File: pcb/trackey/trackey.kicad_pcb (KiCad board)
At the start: 2 copper layers, 55.9 x 77.5 mm, 31 parts, among them J1 trackball_port, J2 Audio-Jack-4, J3 COL_port, J4 ROW_port, J6 has_trackball, J7 is_left, U1 Arduino_Pro_Micro, U2 Arduino_Pro_Micro, U3 MCP23S17

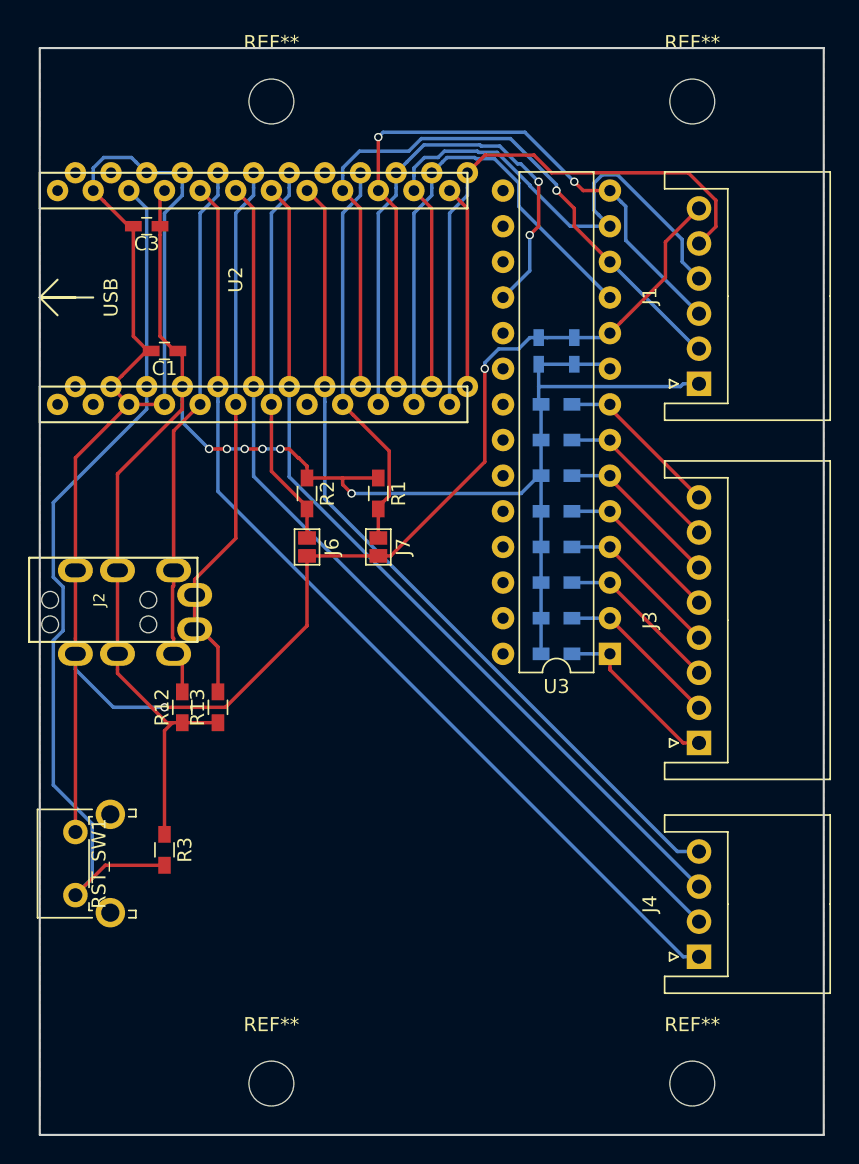
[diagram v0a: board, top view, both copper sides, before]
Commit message: improve pcb size
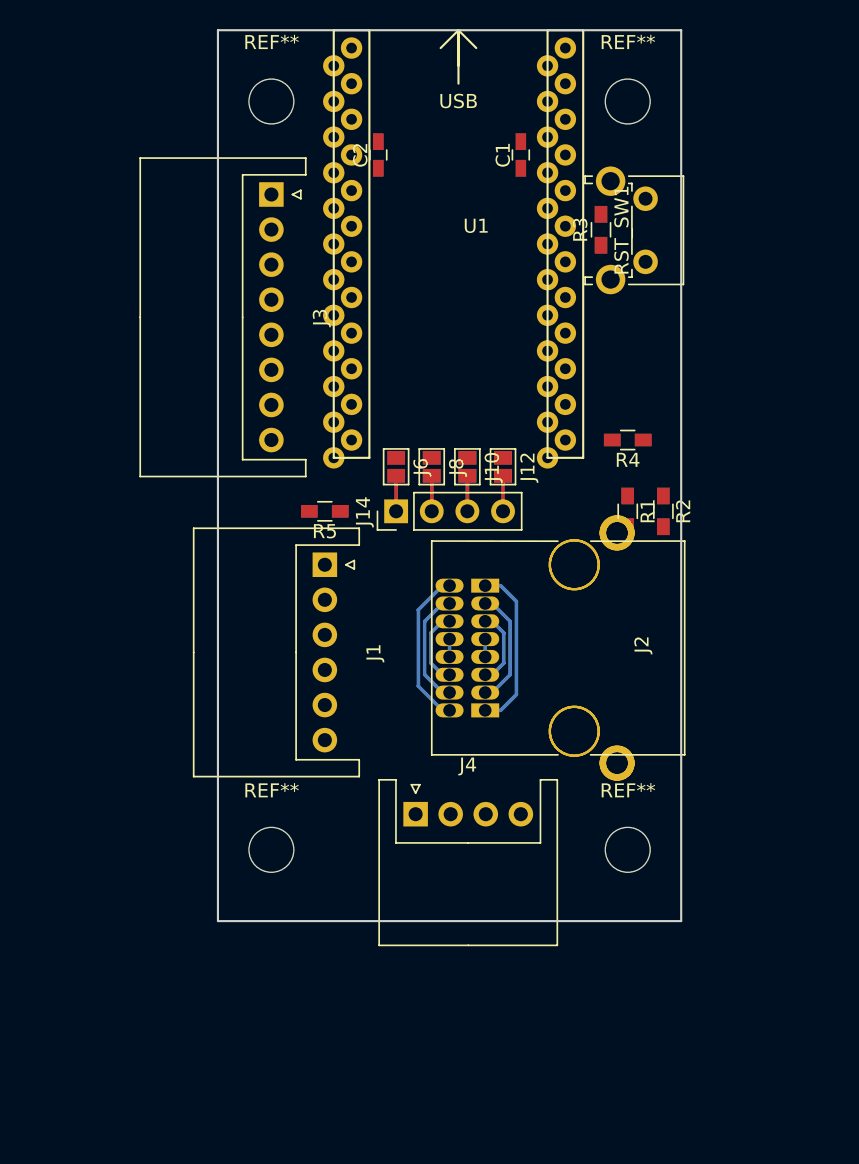
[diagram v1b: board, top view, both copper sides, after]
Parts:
- removed C3: 1uF, Capacitors_SMD:C_0603_HandSoldering
- removed C4: 0.1uF, Capacitors_SMD:C_0603_HandSoldering
- removed R10, R11, R6, R7, R8, R9: 10kΩ, Resistors_SMD:R_0603_HandSoldering
- removed R12, R13: 2.2kΩ, Resistors_SMD:R_0603_HandSoldering
- removed the REF** at (30.0, 0.00)
- removed the REF** at (0.00, 70.0)
- removed the REF** at (30.0, 70.0)
- removed U3: MCP23S17, Housings_DIP:DIP-28_W7.62mm
- added J10: is_left, Connectors:GS2, F.Cu at (14.0, 26.0)
- added J11: is_right, Connectors:GS2, B.Cu at (14.0, 26.0)
- added J12: is_left, Connectors:GS2, F.Cu at (16.5, 26.0)
- added J13: is_right, Connectors:GS2, B.Cu at (16.5, 26.0)
- added J14: OLED_conn, Socket_Strips:Socket_Strip_Straight_1x04_Pitch2.54mm, F.Cu at (8.89, 29.2)
- added J5: RJ45, trackey:RJ45_8, B.Cu at (15.2, 34.5)
- added J8: is_left, Connectors:GS2, F.Cu at (11.4, 26.0)
- added J9: is_right, Connectors:GS2, B.Cu at (11.4, 26.0)
- added REF**: MountingHole_3.2mm_M3, Mounting_Holes:MountingHole_3.2mm_M3, F.Cu at (25.4, 0.00)
- added REF**: MountingHole_3.2mm_M3, Mounting_Holes:MountingHole_3.2mm_M3, F.Cu at (0.00, 53.3)
- added REF**: MountingHole_3.2mm_M3, Mounting_Holes:MountingHole_3.2mm_M3, F.Cu at (25.4, 53.3)
- C2, U1: moved to F.Cu
- J2: value Audio-Jack-4 -> RJ45; footprint trackey:MJ-4PP-9_rev2 -> trackey:RJ45_8
- J6: value has_trackball -> is_left
- J7: value is_left -> is_right; moved to B.Cu
- R1, R2: value 2.2kΩ -> 2.2k
- R4, R5: value 10kΩ -> 2.2k; moved to F.Cu
- U2: moved to B.Cu
- moved RST_SW1 64.2 mm to (26.7, 6.93), turned to 270 degrees
- moved R3 54.1 mm to (23.5, 9.14), turned to 90 degrees
- moved J3 49.6 mm to (0.00, 6.63), turned to 270 degrees
- moved J2 33.5 mm to (15.2, 43.4)
- moved J1 29.6 mm to (3.81, 33.0), turned to 270 degrees
- moved C1 29.0 mm to (17.8, 3.81), turned to 90 degrees
- moved R2 25.4 mm to (27.9, 29.2)
- moved J4 22.6 mm to (10.3, 50.8), turned to 0 degrees
- moved R5 18.2 mm to (3.81, 29.2), turned to 180 degrees
- moved C2 18.1 mm to (7.62, 3.81)
- moved R1 17.8 mm to (25.4, 29.2)
- moved R4 16.1 mm to (25.4, 24.1), turned to 180 degrees
- moved U1 15.1 mm to (14.6, 10.2), turned to 0 degrees
- moved U2 12.1 mm to (10.8, 11.4), turned to 180 degrees
- moved J6 8.54 mm to (8.89, 26.0)
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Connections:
- J2 pad 1: /SCL -> +5V
- J2 pad 3: +5V -> /SCL
- J2 pad 4: GND -> /SCLK
- J3 pad 8: /COL7 -> Net-(J3-Pad8)
- J6 pad 1: /has_trackball -> /SDA
- J6 pad 2: GND -> /OLED_1
- J7 pad 1: /is_left -> GND
- J7 pad 2: GND -> /OLED_1
- R1 pad 2: /is_left -> /SCL
- R2 pad 2: /has_trackball -> /SDA
- R4 pad 2: /COL0 -> Net-(R4-Pad2)
- R5 pad 1: +5V -> GND
- R5 pad 2: /COL1 -> Net-(R5-Pad2)
- U1 pad 1: Net-(U1-Pad1) -> /COL0
- U1 pad 10: /Key_IO_RST -> /COL5
- U1 pad 11: /Key_SS -> /COL6
- U1 pad 13: /Arduino_SS -> Net-(R4-Pad2)
- U1 pad 2: Net-(U1-Pad2) -> /COL1
- U1 pad 7: /has_trackball -> /COL2
- U1 pad 8: Net-(U1-Pad8) -> /COL3
- U1 pad 9: /is_left -> /COL4
- U2 pad 1: Net-(U2-Pad1) -> /COL0
- U2 pad 10: /Key_IO_RST -> /COL5
- U2 pad 11: /Key_SS -> /COL6
- U2 pad 13: /Arduino_SS -> Net-(R5-Pad2)
- U2 pad 2: Net-(U2-Pad2) -> /COL1
- U2 pad 7: /has_trackball -> /COL2
- U2 pad 8: Net-(U2-Pad8) -> /COL3
- U2 pad 9: /is_left -> /COL4
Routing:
- net GND: track 149.5 -> 11.3 mm, vias 2 -> 0
- net +5V: track 125.5 -> 12.0 mm, vias 6 -> 0
- net /ROW0: track 70.0 -> 0.00 mm
- net /ROW1: track 65.8 -> 0.00 mm
- net /RST: track 63.0 -> 0.00 mm
- net /ROW2: track 62.2 -> 0.00 mm
- net /ROW3: track 59.6 -> 0.00 mm
- net /SCLK: track 49.6 -> 1.27 mm, vias 1 -> 0
- net /MISO: track 48.1 -> 1.27 mm, vias 2 -> 0
- net /MOSI: track 48.1 -> 5.49 mm
- net /Key_IO_RST: track 38.4 -> 0.00 mm, vias 2 -> 0
- net /Key_SS: track 35.3 -> 0.00 mm
- net /SCL: track 39.7 -> 5.49 mm
- net /Trackball_SS: track 40.2 -> 8.41 mm
- net /SDA: track 38.6 -> 8.41 mm
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- removed copper zone on B.Cu, net GND
- removed copper zone on F.Cu, net GND
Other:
- board size 55.9 x 77.5 mm -> 33 x 63.5 mm

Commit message: wiring
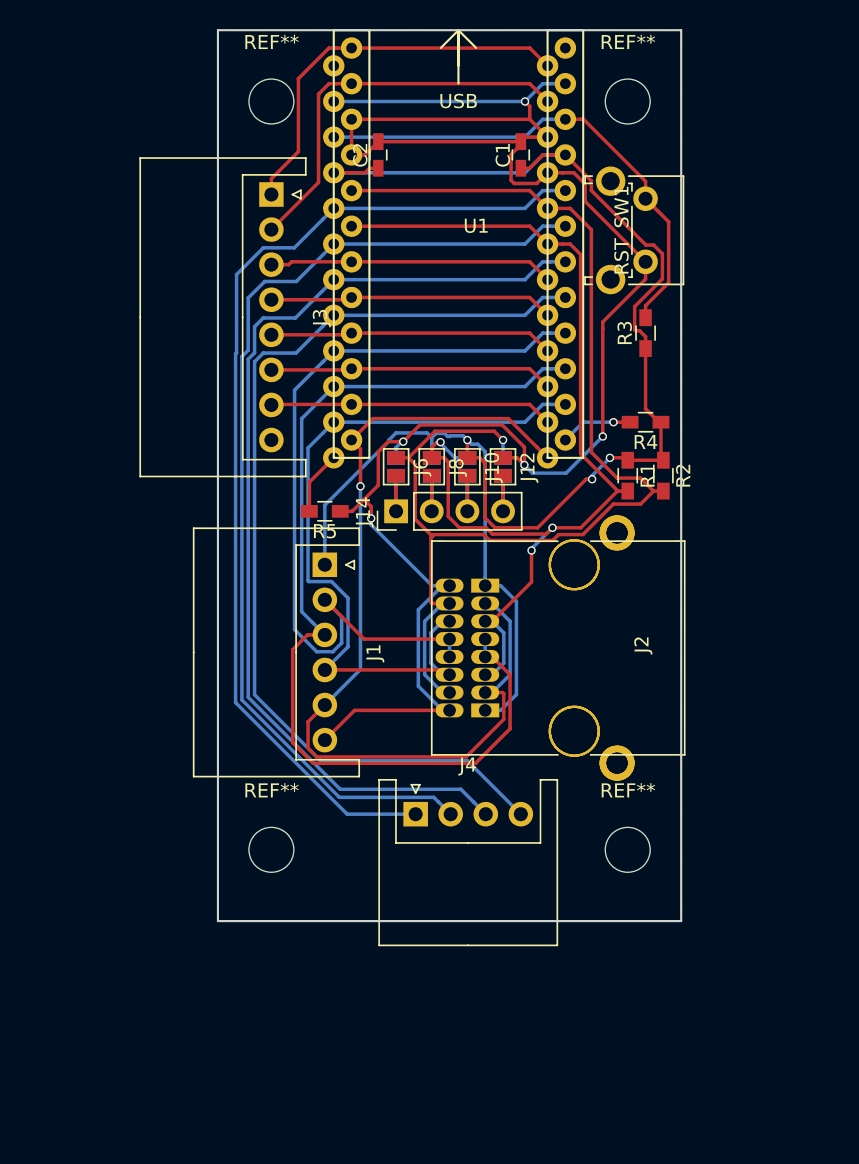
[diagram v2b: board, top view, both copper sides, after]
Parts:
- moved R3 8.02 mm to (26.7, 16.5)
- moved R1 2.54 mm to (25.4, 26.7)
- moved R2 2.54 mm to (27.9, 26.7)
- moved R4 1.80 mm to (26.7, 22.9)
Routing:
- net GND: track 11.3 -> 139.8 mm, vias 0 -> 5
- net +5V: track 12.0 -> 114.4 mm, vias 0 -> 3
- net /SDA: track 8.41 -> 88.6 mm, vias 0 -> 1
- net /ROW0: track 0.00 -> 72.6 mm
- net /ROW1: track 0.00 -> 71.8 mm
- net /ROW2: track 0.00 -> 71.1 mm
- net /ROW3: track 0.00 -> 70.3 mm
- net /MISO: track 1.27 -> 70.3 mm
- net /SCL: track 5.49 -> 73.3 mm, vias 0 -> 3
- net /Trackball_SS: track 8.41 -> 66.5 mm, vias 0 -> 1
- net /SCLK: track 1.27 -> 57.2 mm
- net /MOSI: track 5.49 -> 52.8 mm
- net /RST: track 0.00 -> 35.7 mm
- net /COL0: track 0.00 -> 28.2 mm
- net /COL1: track 0.00 -> 28.2 mm
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- added copper zone on B.Cu, net GND
- added copper zone on F.Cu, net GND
